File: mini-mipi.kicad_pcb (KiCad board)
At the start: 4 copper layers, 43.2 x 34.9 mm, 56 parts, among them IC1 ECP5-BGA256, J1 Conn_ARM_JTAG_SWD_10, J2 Conn_01x15, J3 USB_B_Micro, J4 Micro_SD_Card, U1 TPS74633, U2 TPS74618, U3 TPS74625, U4 TPS74611, U5 AT25SF081-SSHD-X, U6 S27KL0641, U7 OSC_25M

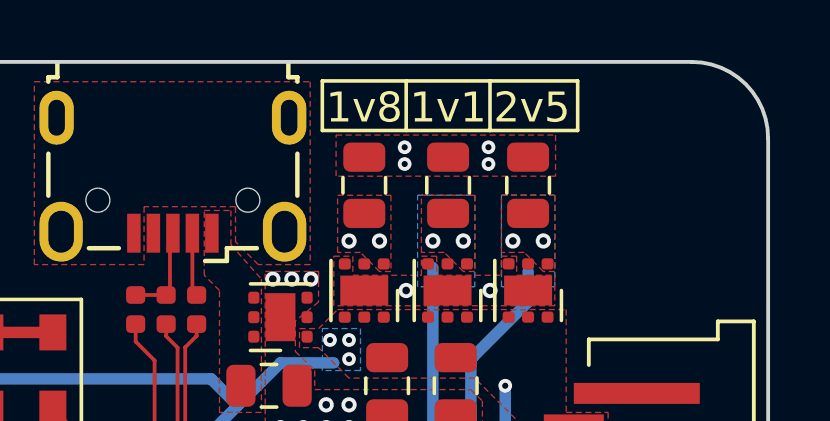
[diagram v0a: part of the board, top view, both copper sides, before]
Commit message: Change box around voltage labels
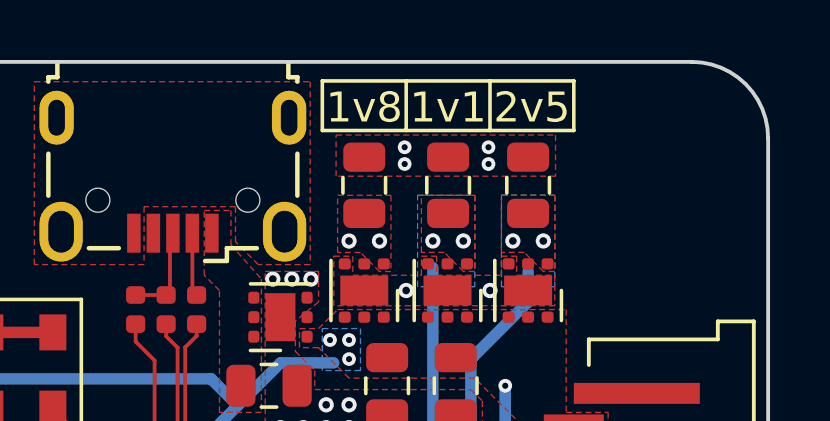
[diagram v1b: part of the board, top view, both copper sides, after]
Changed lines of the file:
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@@
   (general
     (thickness 1.6)
-    (drawings 17)
+    (drawings 20)
     (tracks 1149)
     (modules 56)
@@
     )
   )
+  (gr_line (start 169.926 64.516) (end 169.926 62.865) (layer "F.SilkS") (width 0.12))
+  (gr_line (start 178.308 64.516) (end 169.926 64.516) (layer "F.SilkS") (width 0.12))
+  (gr_line (start 178.308 62.865) (end 178.308 64.516) (layer "F.SilkS") (width 0.12))
+  (gr_line (start 169.926 62.865) (end 178.308 62.865) (layer "F.SilkS") (width 0.12))
   (gr_text "Mini-Mipi\n${GIT_REV}\nUNTESTED" (at 145.034 86.995 270) (layer "B.SilkS")
     (effects (font (size 1 1) (thickness 0.15)) (justify mirror))
@@
   (gr_line (start 172.72 62.865) (end 172.72 64.516) (layer "F.SilkS") (width 0.12))
   (gr_line (start 175.514 64.516) (end 175.514 62.865) (layer "F.SilkS") (width 0.12))
-  (gr_rect (start 169.926 62.865) (end 178.435 64.516) (layer "F.SilkS") (width 0.12))
   (gr_text "2v5" (at 176.911 63.754) (layer "F.SilkS")
     (effects (font (size 1 1) (thickness 0.15)))
